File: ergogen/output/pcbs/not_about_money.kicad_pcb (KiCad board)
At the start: 2 copper layers, 118 x 80 mm, 57 parts

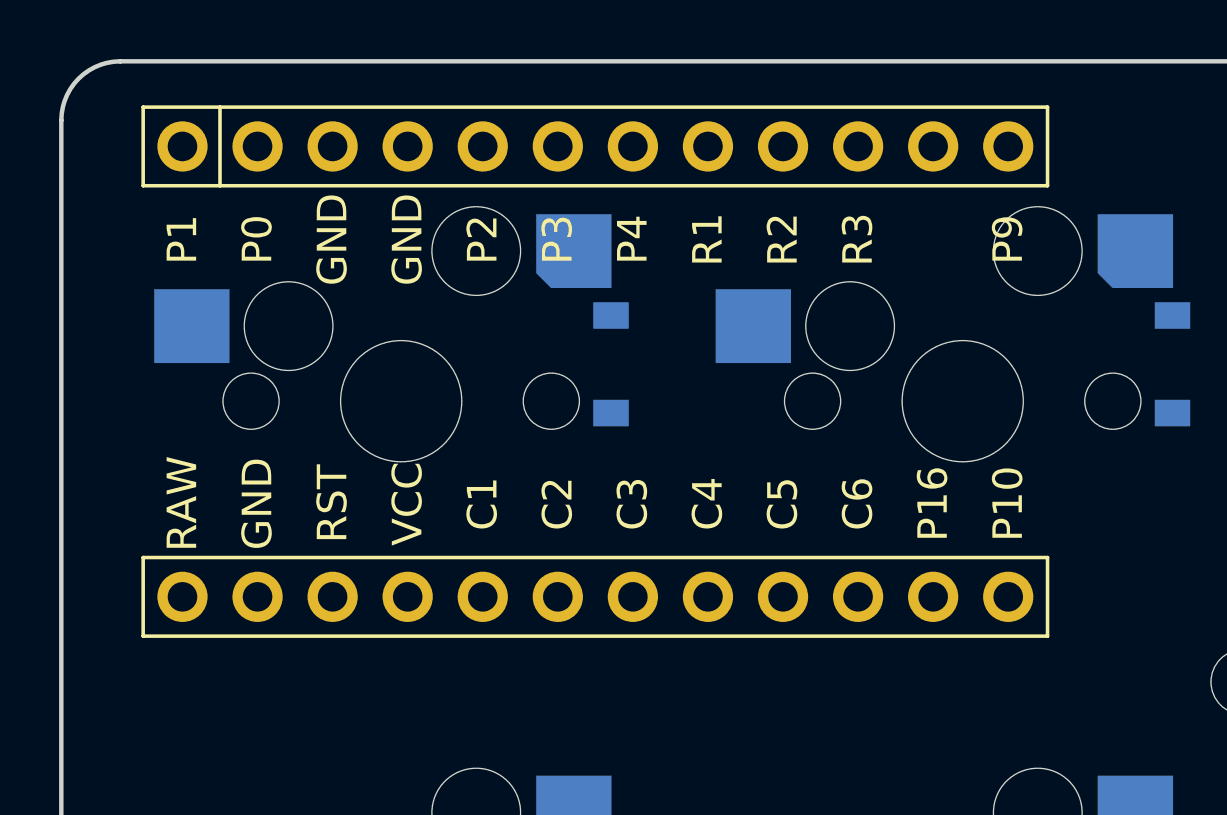
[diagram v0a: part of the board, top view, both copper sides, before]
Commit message: Update assets
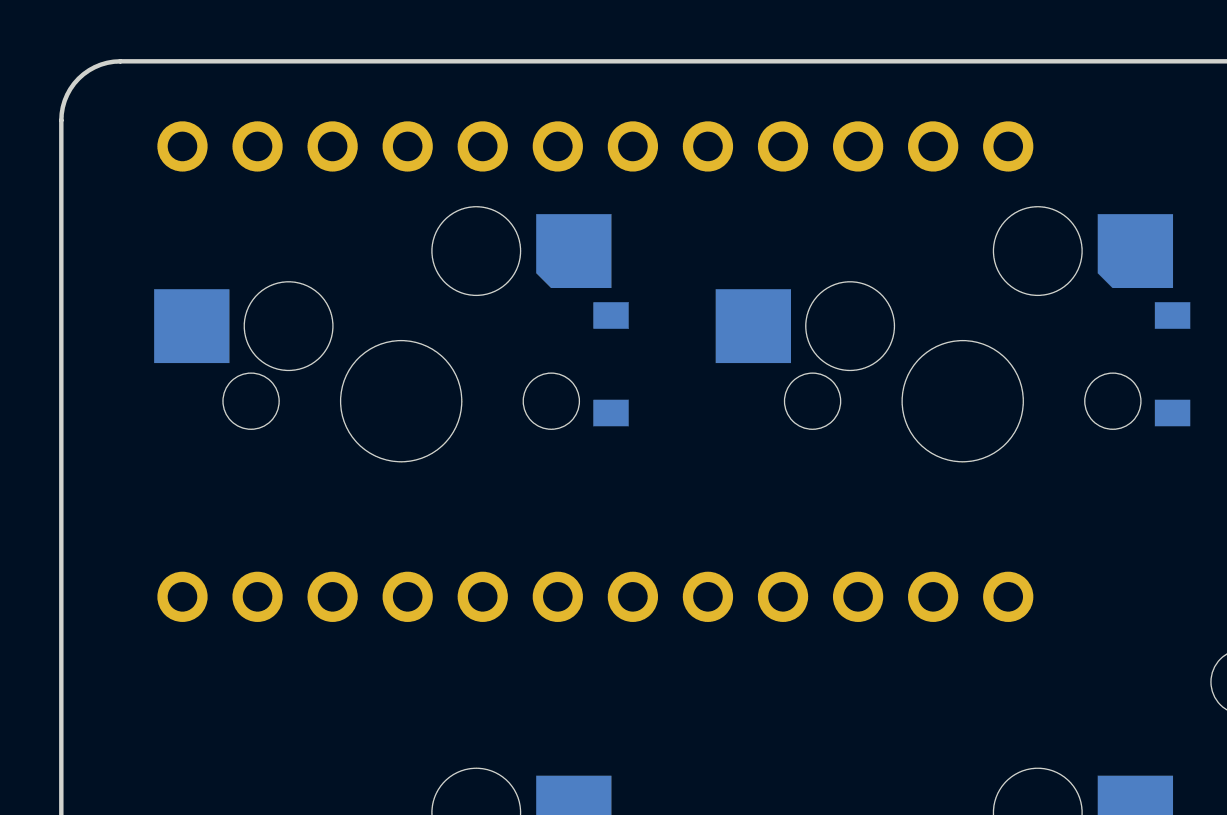
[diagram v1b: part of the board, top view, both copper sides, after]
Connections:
- MCU1 pad 13: P10 -> R2
- MCU1 pad 14: P16 -> R1
- MCU1 pad 8: R1 -> P5
- MCU1 pad 9: R2 -> P6

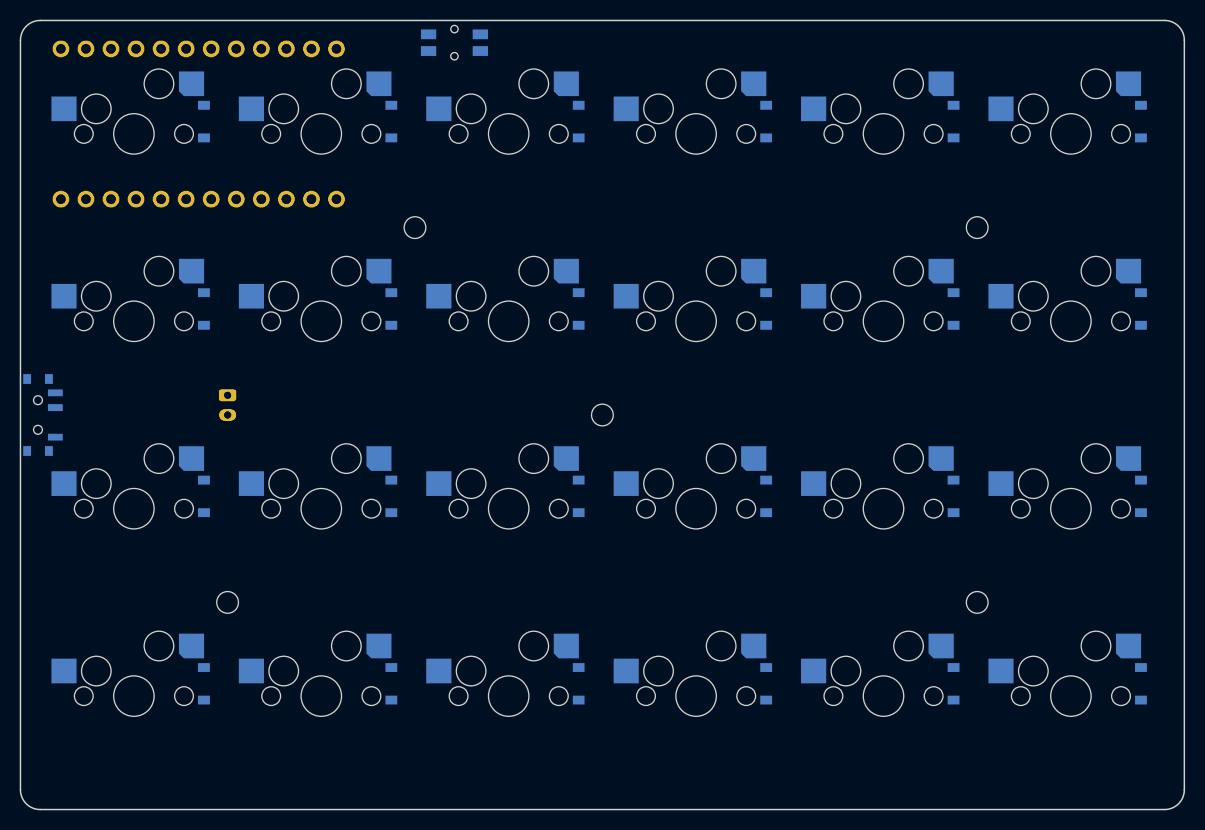
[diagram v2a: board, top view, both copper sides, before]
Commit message: Update assets
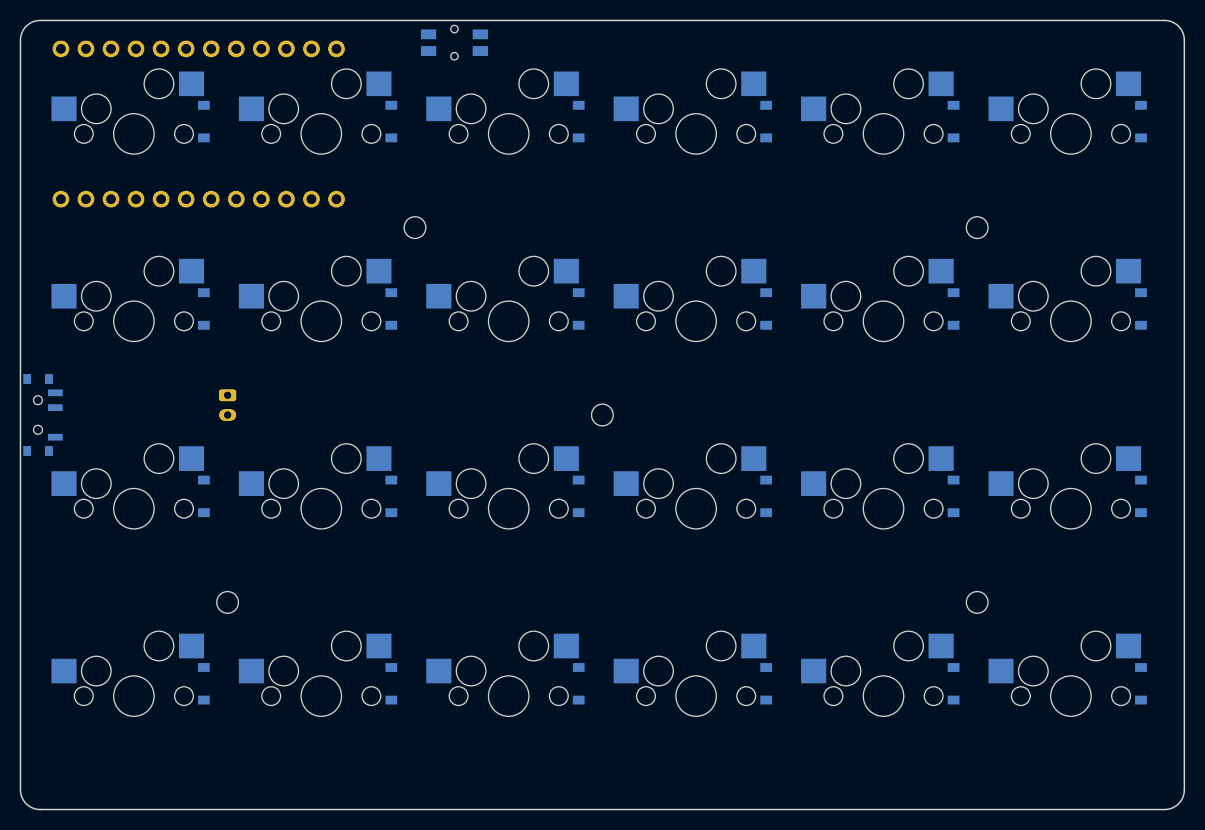
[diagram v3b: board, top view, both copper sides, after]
